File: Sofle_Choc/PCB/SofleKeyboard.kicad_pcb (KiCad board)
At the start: 2 copper layers, 143.4 x 111.8 mm, 88 parts, among them J2 4PIN, J3 OLED, P1 i2c_pin, P2 i2c_pin, SW1 SW_PUSH_LED, SW10 SW_PUSH_LED, SW11 SW_PUSH_LED, SW12 SW_PUSH_LED, SW13 SW_PUSH_LED, SW14 SW_PUSH_LED, SW15 SW_PUSH_LED, SW16 SW_PUSH_LED, SW17 SW_PUSH_LED, SW18 SW_PUSH_LED, SW19 SW_PUSH_LED, SW2 SW_PUSH_LED, SW20 SW_PUSH_LED, SW21 SW_PUSH_LED, SW22 SW_PUSH_LED, SW23 SW_PUSH_LED, SW24 SW_PUSH_LED, SW25 Rotary_Encoder_Switch, SW26 SW_PUSH_LED, SW27 SW_PUSH_LED, SW28 SW_PUSH_LED, SW29 SW_PUSH_LED, SW3 SW_PUSH_LED, SW30 SW_PUSH_LED, SW4 SW_PUSH_LED, SW5 SW_PUSH_LED, SW6 SW_PUSH_LED, SW7 SW_PUSH_LED, SW8 SW_PUSH_LED, SW9 SW_PUSH_LED, U1 ProMicro

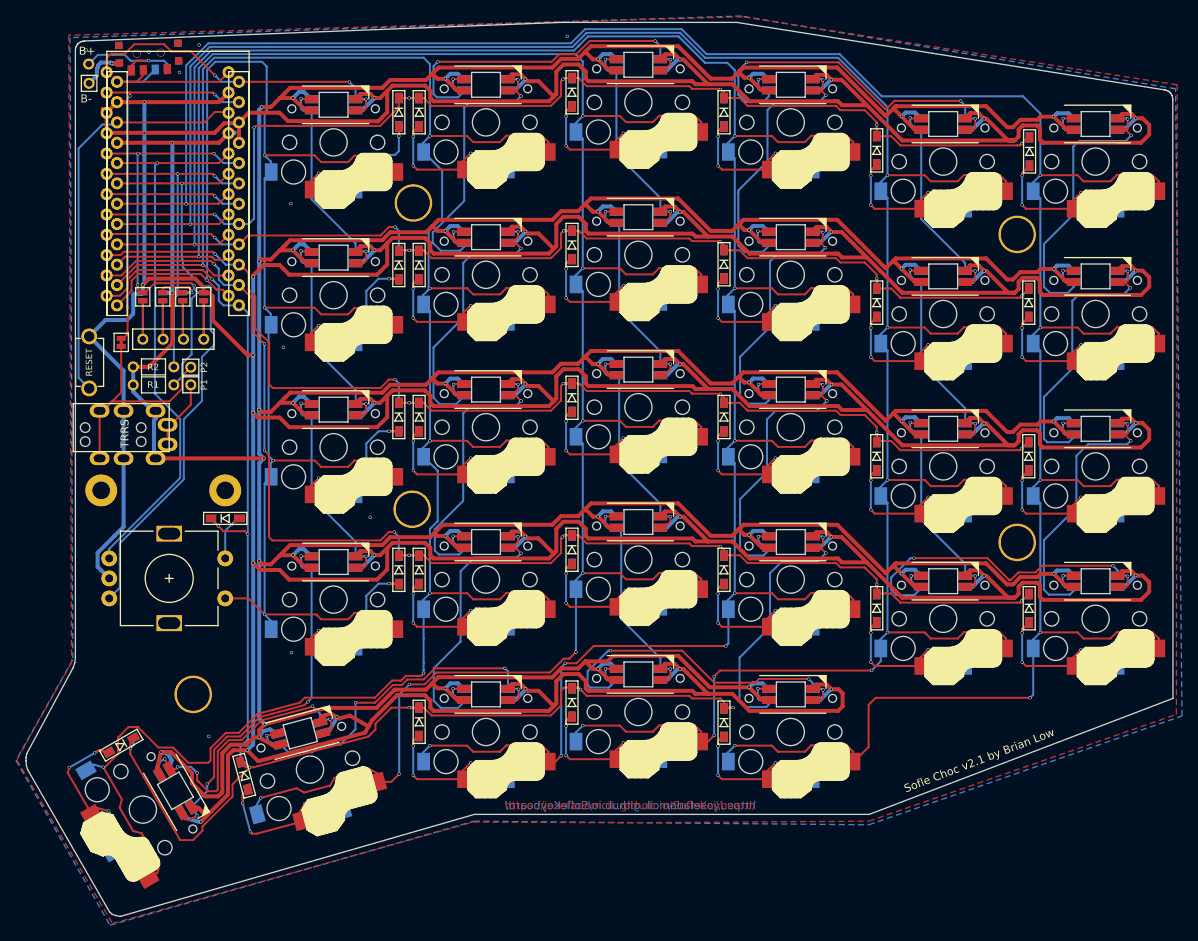
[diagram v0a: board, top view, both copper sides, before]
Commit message: Minimum to meet AllPcb freebie size
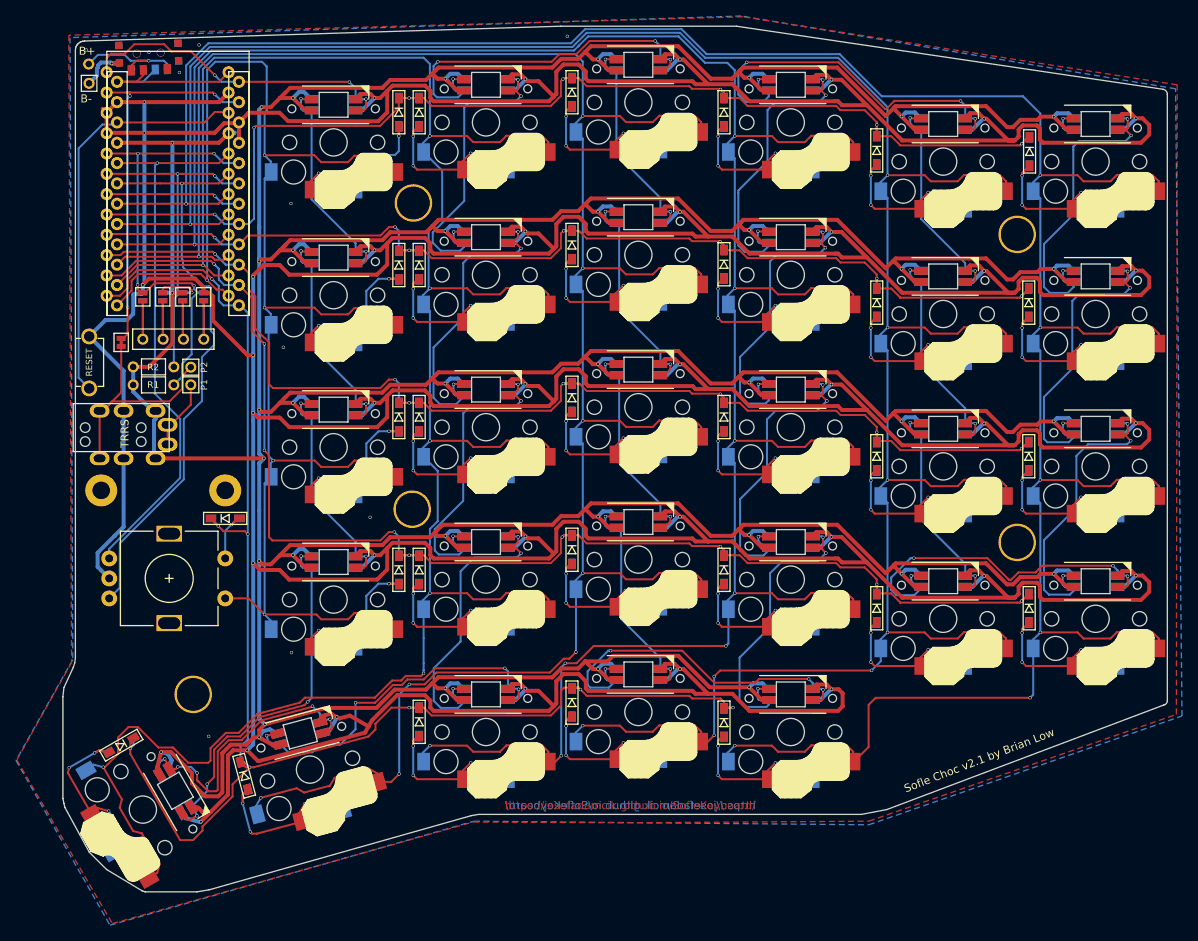
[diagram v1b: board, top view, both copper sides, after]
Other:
- board size 143.4 x 111.8 mm -> 138 x 108.2 mm
